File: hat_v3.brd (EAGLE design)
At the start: 65 x 56.5 mm, 42 parts, among them U1 ADS1115IDGST, U2 ADXL345, U5 MCP2515-I/SO, U6 MCP2551, X1 16Mhz

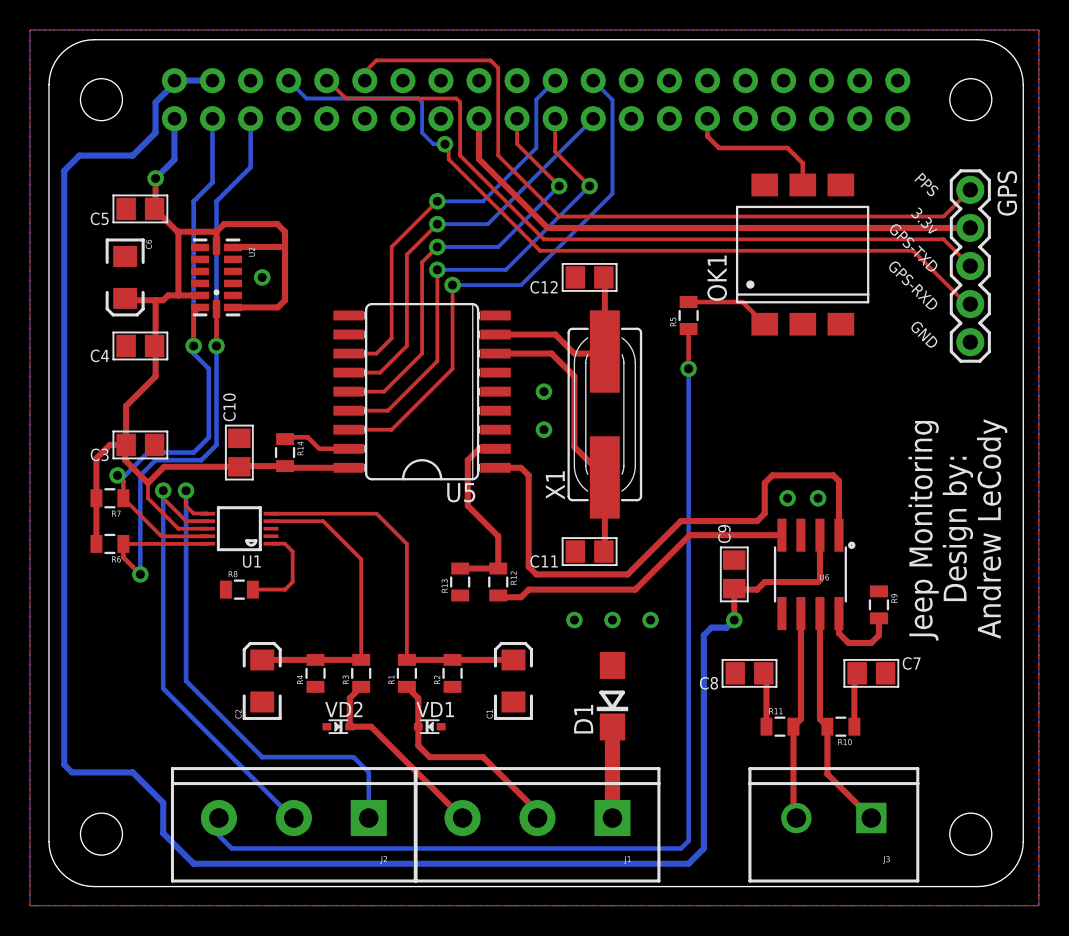
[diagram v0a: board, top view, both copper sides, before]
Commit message: Reworked v3
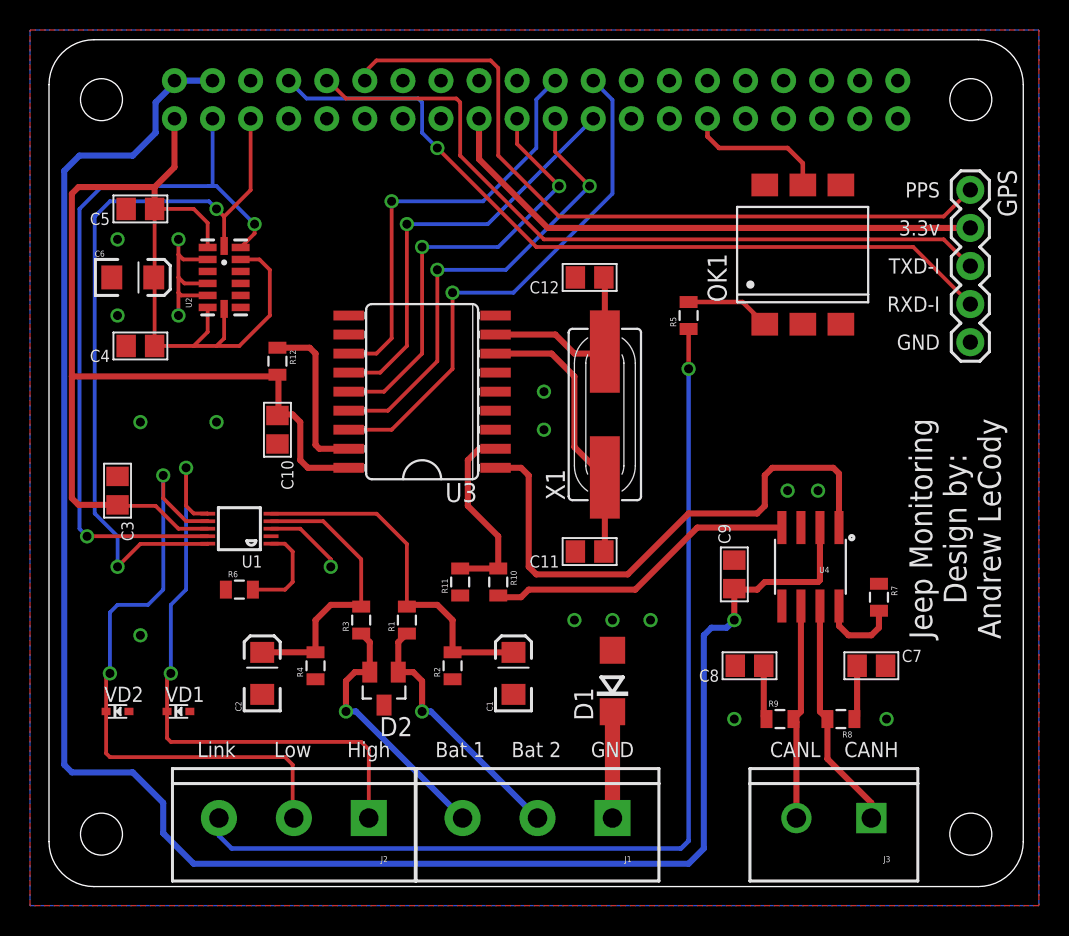
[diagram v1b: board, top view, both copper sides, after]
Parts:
- removed R13: 22k, SparkFun-Passives:0805
- removed R14: 4k7, SparkFun-Passives:0805
- removed U6: MCP2551, SparkFun-DigitalIC:SO08
- added D2: (no value), diode:SOT23
- added U4: MCP2551, SparkFun-DigitalIC:SO08
- C1, C2: value 100uF -> 10uF; device SparkFun:EIA3216 -> SparkFun-Capacitors:EIA3216
- C10: value 100nF -> 0.1uF
- C6: device SparkFun:EIA3216 -> SparkFun-Capacitors:EIA3216
- R10: value 100 -> 10k
- R11: value 100 -> 22k
- R12, R7: value 10k -> 4k7
- R8: value 10k -> 100
- R9: value 4k7 -> 100
- VD1, VD2: device diode:SOD523@1 -> diode:SOD523
- moved R7 51.7 mm to (55.4, 19.3), turned to 270 degrees
- moved R8 41.1 mm to (52.8, 11.2), turned to 180 degrees
- moved R10 24.8 mm to (30.0, 20.3), turned to 270 degrees
- moved R11 23.4 mm to (27.4, 20.3), turned to 90 degrees
- moved R12 20.8 mm to (15.2, 35.1)
- moved VD1 16.8 mm to (8.64, 11.7)
- moved VD2 14.8 mm to (4.57, 11.7), turned to 0 degrees
- moved R9 10.1 mm to (48.8, 11.2), turned to 0 degrees
- moved R6 9.16 mm to (12.7, 19.8), turned to 0 degrees
- moved R1 3.56 mm to (23.9, 17.8)
- moved R3 3.56 mm to (20.8, 17.8)
- moved C3 3.41 mm to (4.57, 26.4), turned to 270 degrees
- moved C10 2.96 mm to (15.2, 30.5), turned to 270 degrees
- moved D1 1.02 mm to (37.6, 13.7)
- moved C1 0.51 mm to (31.0, 14.2)
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- renumbered U5 to U3
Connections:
- net 3.3V: now also R12.2; no longer R14.2, R6.2, R7.2
- net 5V: now also U4.2; no longer U6.2
- net ADDR: now also R6.2; no longer R8.2
- net BAT-1-INPUT: now also D2.1; no longer VD1.C
- net BAT-2-INPUT: now also D2.2; no longer VD2.C
- net CANH: now also R8.2, U4.7; no longer R10.2, U6.7
- net CANL: now also R9.2, U4.6; no longer R11.2, U6.6
- net GND: now also D2.3, R11.1, R6.1, R7.1, U4.3; no longer R13.1, R8.1, R9.1, U6.3
- net N$4: now also R10.1, R11.2; no longer R12.1, R13.2
- net N$5: now also R7.2, U4.8; no longer R9.2, U6.8
- net N$6: now also R8.1; no longer R10.1
- net N$8: now also R9.1; no longer R11.1
- net RXCAN: now also R10.2, U4.4; no longer R12.2, U6.4
- net SCL: no longer R6.1
- net SDA: no longer R7.1
- net SHUNT-HIGH-INPUT: now also VD1.C
- net SHUNT-LOW-INPUT: now also VD2.C
- net TXCAN: now also U4.1; no longer U6.1
- net U5_RST: now also R12.1; no longer R14.1
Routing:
- net 3.3V: track 117.5 -> 138.4 mm, vias 1 -> 0
- net GND: track 0.00 -> 16.6 mm, vias 8 -> 17
- net SHUNT-LOW-INPUT: track 29.6 -> 42.8 mm, vias 1 -> 2
- net SDA: track 40.5 -> 49.9 mm
- net SHUNT-HIGH-INPUT: track 33.1 -> 41.1 mm, vias 1 -> 2
- net U5_RST: track 4.61 -> 11.1 mm
- net BAT-2-INPUT: track 13.0 -> 17.4 mm, vias 0 -> 1
- net SCL: track 45.8 -> 49.4 mm
- net BAT-1-INPUT: track 14.4 -> 17.3 mm, vias 0 -> 1
- net GPIO25: track 26.8 -> 28.6 mm
- net SPI_SCLK: track 26.9 -> 28.1 mm
- net N$1: track 6.08 -> 7.09 mm
- net BAT-2: track 20.4 -> 19.5 mm
- net BAT-1: track 24.7 -> 23.8 mm
- net SPI_MOSI: track 29.0 -> 29.5 mm
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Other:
- board text added: "Bat 1"
- board text added: "Bat 2"
- board text added: "CANH"
- board text added: "CANL"
- board text added: "High"
- board text added: "Link"
- board text added: "Low"
- board text added: "RXD-I"
- board text added: "TXD-I"
- board text removed: "GPS-RXD"
- board text removed: "GPS-TXD"
